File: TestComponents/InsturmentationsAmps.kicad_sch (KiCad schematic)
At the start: 58 parts, among them SW1 SW_DPDT, SW2 SW_DP3T, SW3 SW_DP3T, SW4 SW_DP3T, U13 X, U3 REF200AU, U4 MCP6L01x-xLT, U8 ADR5041B, U9 ADR5044B

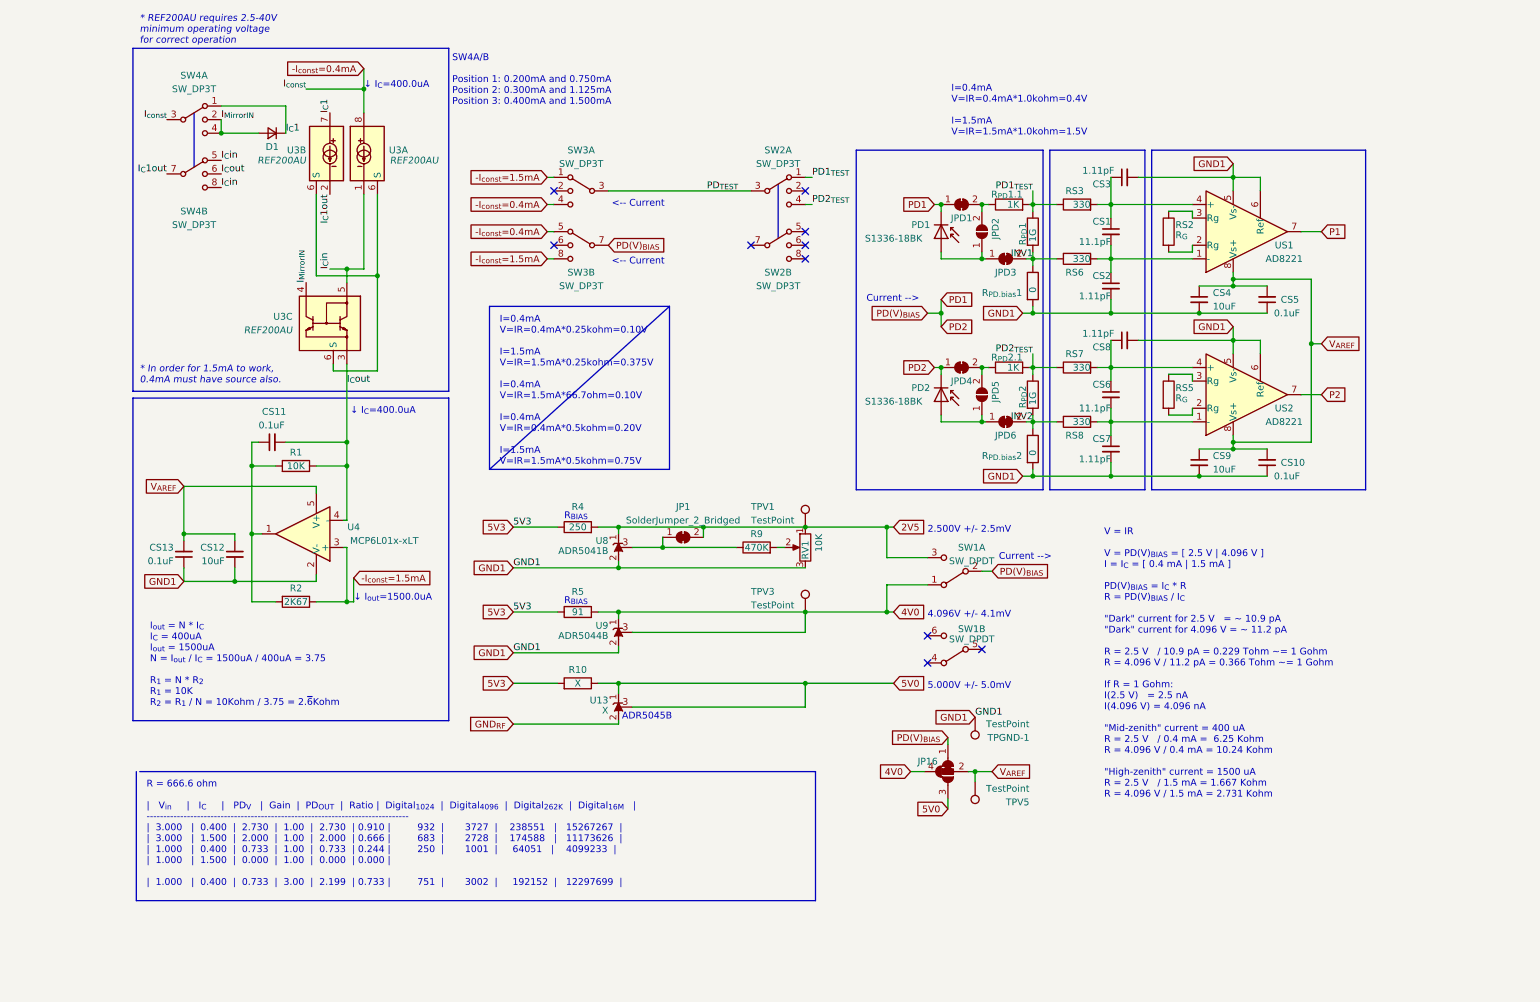
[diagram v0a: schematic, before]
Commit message: SpectDrone Development
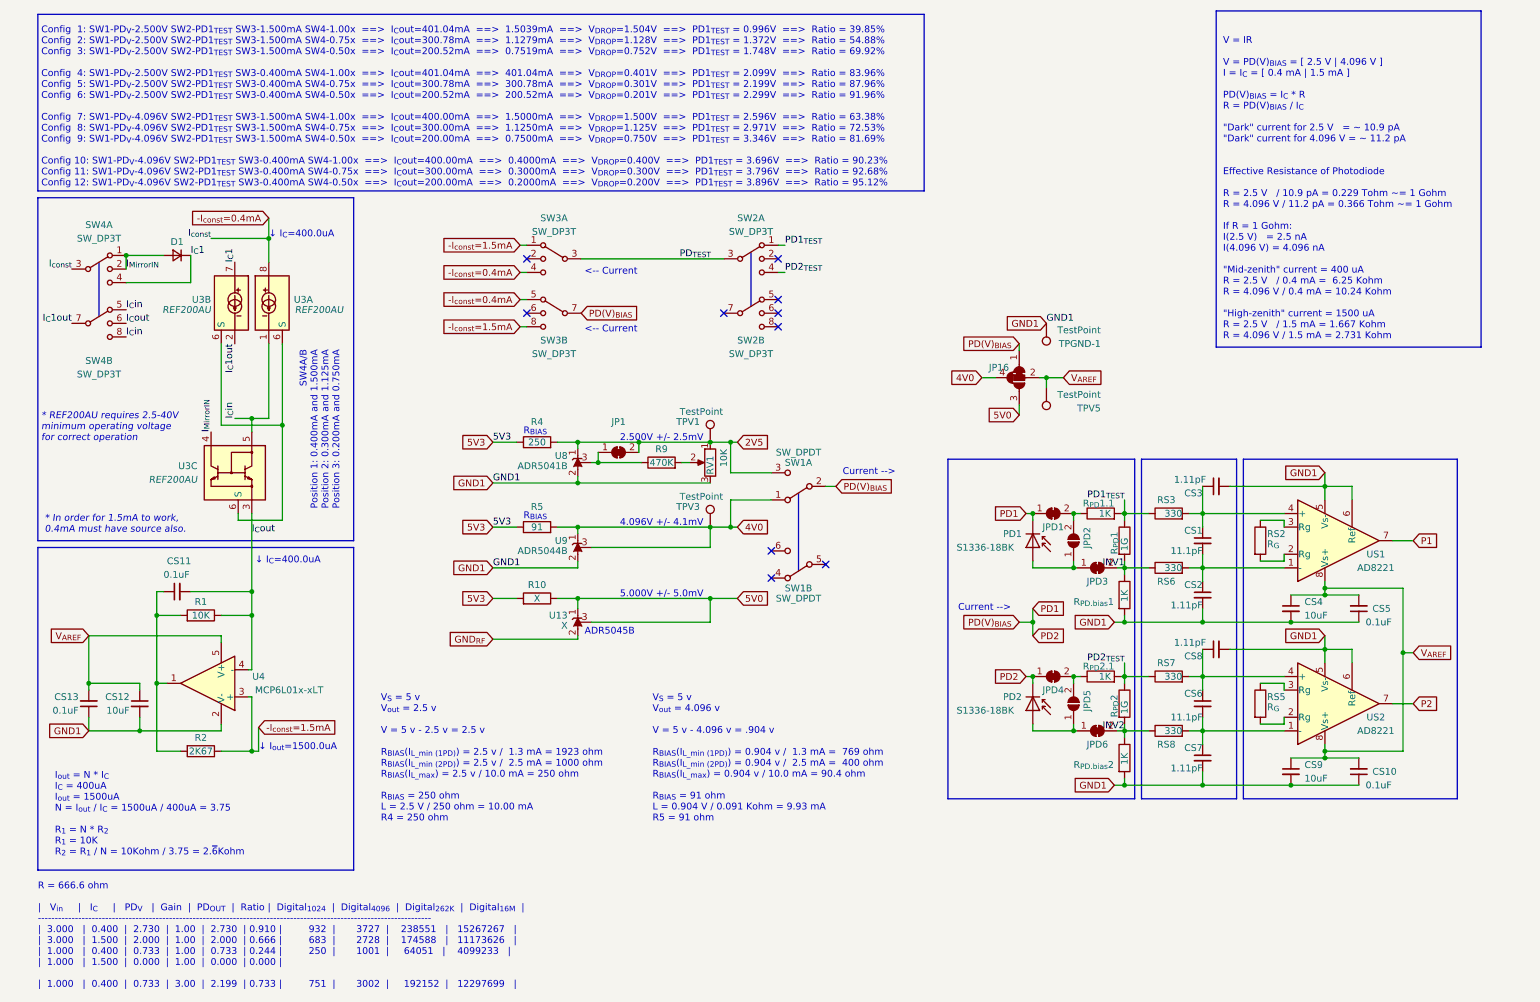
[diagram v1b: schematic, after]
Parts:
- R_{PD.bias}1, R_{PD.bias}2: value 0 -> 1K; Part Number ERJ-6GEY0R00V -> (none)
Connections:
- net I_{C}1: now also SW4.4; no longer SW4.1
- net I_{Mirror}_{IN}: now also SW4.1; no longer SW4.4
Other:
- note added: "Config 1: SW1-PD_{V}-2.500V SW2-PD1_{TEST} SW3-1.500mA SW4-1.00x ==> I_{C}out=401.04mA ==> 1.5039mA ==> V_{DROP}=1.504V ==> PD1_{TEST} = 0.996V ==> Ratio = 39.85% Config 2: SW1-PD_{V}-2.500V SW2-PD1_{TEST} SW3-1.500mA SW4-0.75x ==> I_{C}out=300.78mA ==> 1.1279mA ==> V_{DROP}=1.128V ==> PD1_{TEST} = 1.372V ==> Ratio = 54.88% Config 3: SW1-PD_{V}-2.500V SW2-PD1_{TEST} SW3-1.500mA SW4-0.50x ==> I_{C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"
- note added: "R = 666.6 ohm | V_{in} | I_{C} | PD_{V} | Gain | PD_{OUT} | Ratio | Digital_{1024} | Digital_{4096} | Digital_{262K} | Digital_{16M} | --------------------------------------------------------------------------------------------------------------------- | 3.000 | 0.400 | 2.730 | 1.00 | 2.730 | 0.910 | 932 | 3727 | 238551 | 15267267 | | 3.000 | 1.500 | 2.000 | 1.00 | 2.000 | 0.666 | 683 | 2728 | 17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"
- note added: "SW4A/B Position 1: 0.400mA and 1.500mA Position 2: 0.300mA and 1.125mA Position 3: 0.200mA and 0.750mA"
- note added: "V = IR V = PD(V)_{BIAS} = [ 2.5 V | 4.096 V ] I = I_{C} = [ 0.4 mA | 1.5 mA ] PD(V)_{BIAS} = I_{C} * R R = PD(V)_{BIAS} / I_{C} "Dark" current for 2.5 V = ~ 10.9 pA "Dark" current for 4.096 V = ~ 11.2 pA Effective Resistance of Photodiode R = 2.5 V / 10.9 pA = 0.229 Tohm ~= 1 Gohm R = 4.096 V / 11.2 pA = 0.366 Tohm ~= 1 Gohm If R = 1 Gohm: I(2.5 V) = 2.5 nA I(4.096 V) = 4.096 nA "Mid-zenith" curr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"
- note added: "V_{S} = 5 v V_{out} = 2.5 v V = 5 v - 2.5 v = 2.5 v R_{BIAS}(I_{L_min (1PD)}) = 2.5 v / 1.3 mA = 1923 ohm R_{BIAS}(I_{L_min (2PD)}) = 2.5 v / 2.5 mA = 1000 ohm R_{BIAS}(I_{L_max}) = 2.5 v / 10.0 mA = 250 ohm R_{BIAS} = 250 ohm L = 2.5 V / 250 ohm = 10.00 mA R4 = 250 ohm"
- note added: "V_{S} = 5 v V_{out} = 4.096 v V = 5 v - 4.096 v = .904 v R_{BIAS}(I_{L_min (1PD)}) = 0.904 v / 1.3 mA = 769 ohm R_{BIAS}(I_{L_min (2PD)}) = 0.904 v / 2.5 mA = 400 ohm R_{BIAS}(I_{L_max}) = 0.904 v / 10.0 mA = 90.4 ohm R_{BIAS} = 91 ohm L = 0.904 V / 0.091 Kohm = 9.93 mA R5 = 91 ohm"
- note removed: "I=0.4mA V=IR=0.4mA*0.25kohm=0.10V I=1.5mA V=IR=1.5mA*0.25kohm=0.375V I=0.4mA V=IR=1.5mA*66.7ohm=0.10V I=0.4mA V=IR=0.4mA*0.5kohm=0.20V I=1.5mA V=IR=1.5mA*0.5kohm=0.75V"
- note removed: "I=0.4mA V=IR=0.4mA*1.0kohm=0.4V I=1.5mA V=IR=1.5mA*1.0kohm=1.5V"
- note removed: "R = 666.6 ohm | V_{in} | I_{C} | PD_{V} | Gain | PD_{OUT} | Ratio | Digital_{1024} | Digital_{4096} | Digital_{262K} | Digital_{16M} | ------------------------------------------------------------------------------ | 3.000 | 0.400 | 2.730 | 1.00 | 2.730 | 0.910 | 932 | 3727 | 238551 | 15267267 | | 3.000 | 1.500 | 2.000 | 1.00 | 2.000 | 0.666 | 683 | 2728 | 174588 | 11173626 | | 1.000 | 0.400 | 0.7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"
- note removed: "SW4A/B Position 1: 0.200mA and 0.750mA Position 2: 0.300mA and 1.125mA Position 3: 0.400mA and 1.500mA"
- note removed: "V = IR V = PD(V)_{BIAS} = [ 2.5 V | 4.096 V ] I = I_{C} = [ 0.4 mA | 1.5 mA ] PD(V)_{BIAS} = I_{C} * R R = PD(V)_{BIAS} / I_{C} "Dark" current for 2.5 V = ~ 10.9 pA "Dark" current for 4.096 V = ~ 11.2 pA R = 2.5 V / 10.9 pA = 0.229 Tohm ~= 1 Gohm R = 4.096 V / 11.2 pA = 0.366 Tohm ~= 1 Gohm If R = 1 Gohm: I(2.5 V) = 2.5 nA I(4.096 V) = 4.096 nA "Mid-zenith" current = 400 uA R = 2.5 V / 0.4 mA = 6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"
- moved on the sheet: CS1, CS10, CS11, CS12, CS13, CS2, CS3, CS4, CS5, CS6, CS7, CS8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
